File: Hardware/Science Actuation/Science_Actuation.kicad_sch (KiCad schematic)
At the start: 110 parts, among them J2 RJ45_LED_Shielded, Q1 BSS138, Q10 AO3401A, Q9 BSS138, SW1 SW_Push, SW10 SW_SPDT, SW2 SW_Push, SW3 SW_Push, SW4 SW_Push, SW5 SW_Push, SW6 SW_Push, SW7 SW_Push, SW8 SW_Push, SW9 SW_Push, U2 OKI, U2 Teensy4.1_DEV-16771

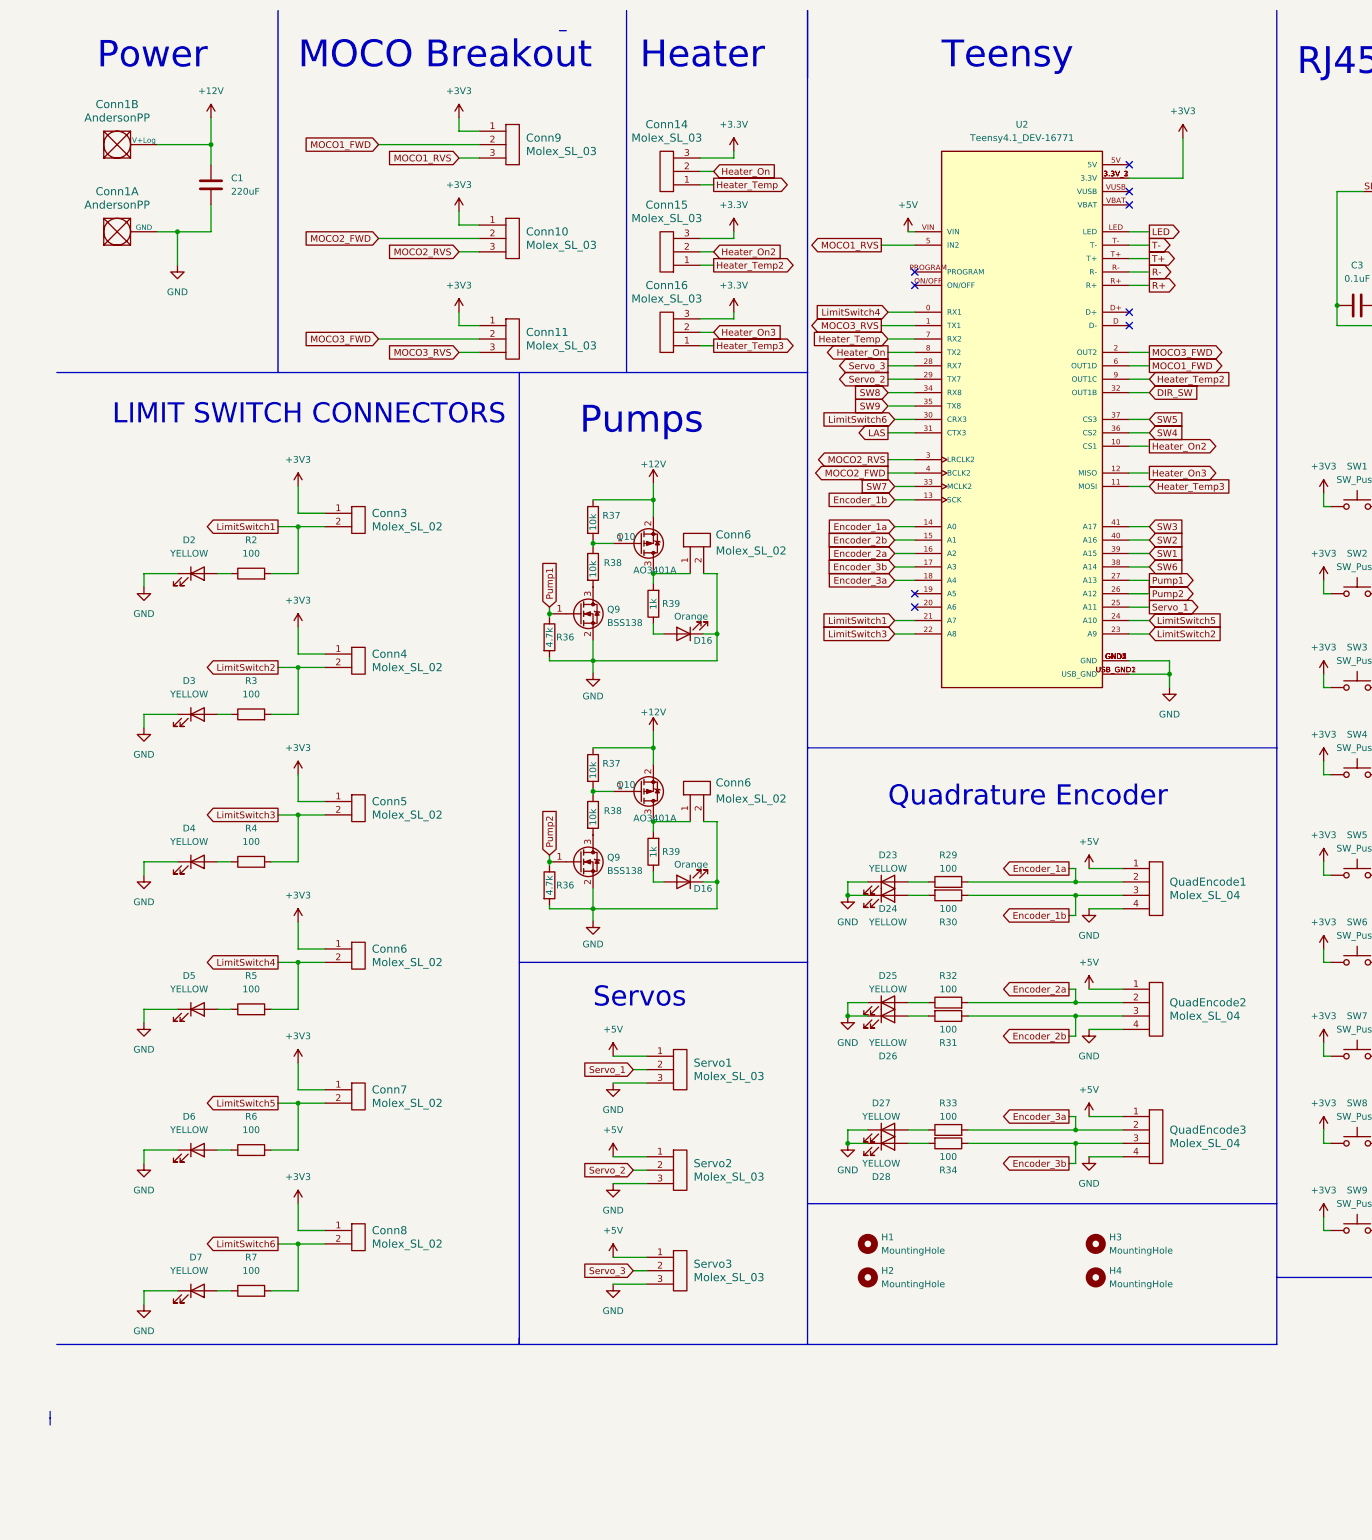
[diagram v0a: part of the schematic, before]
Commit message: Temporary state
Removed things. Added a motor. WIP
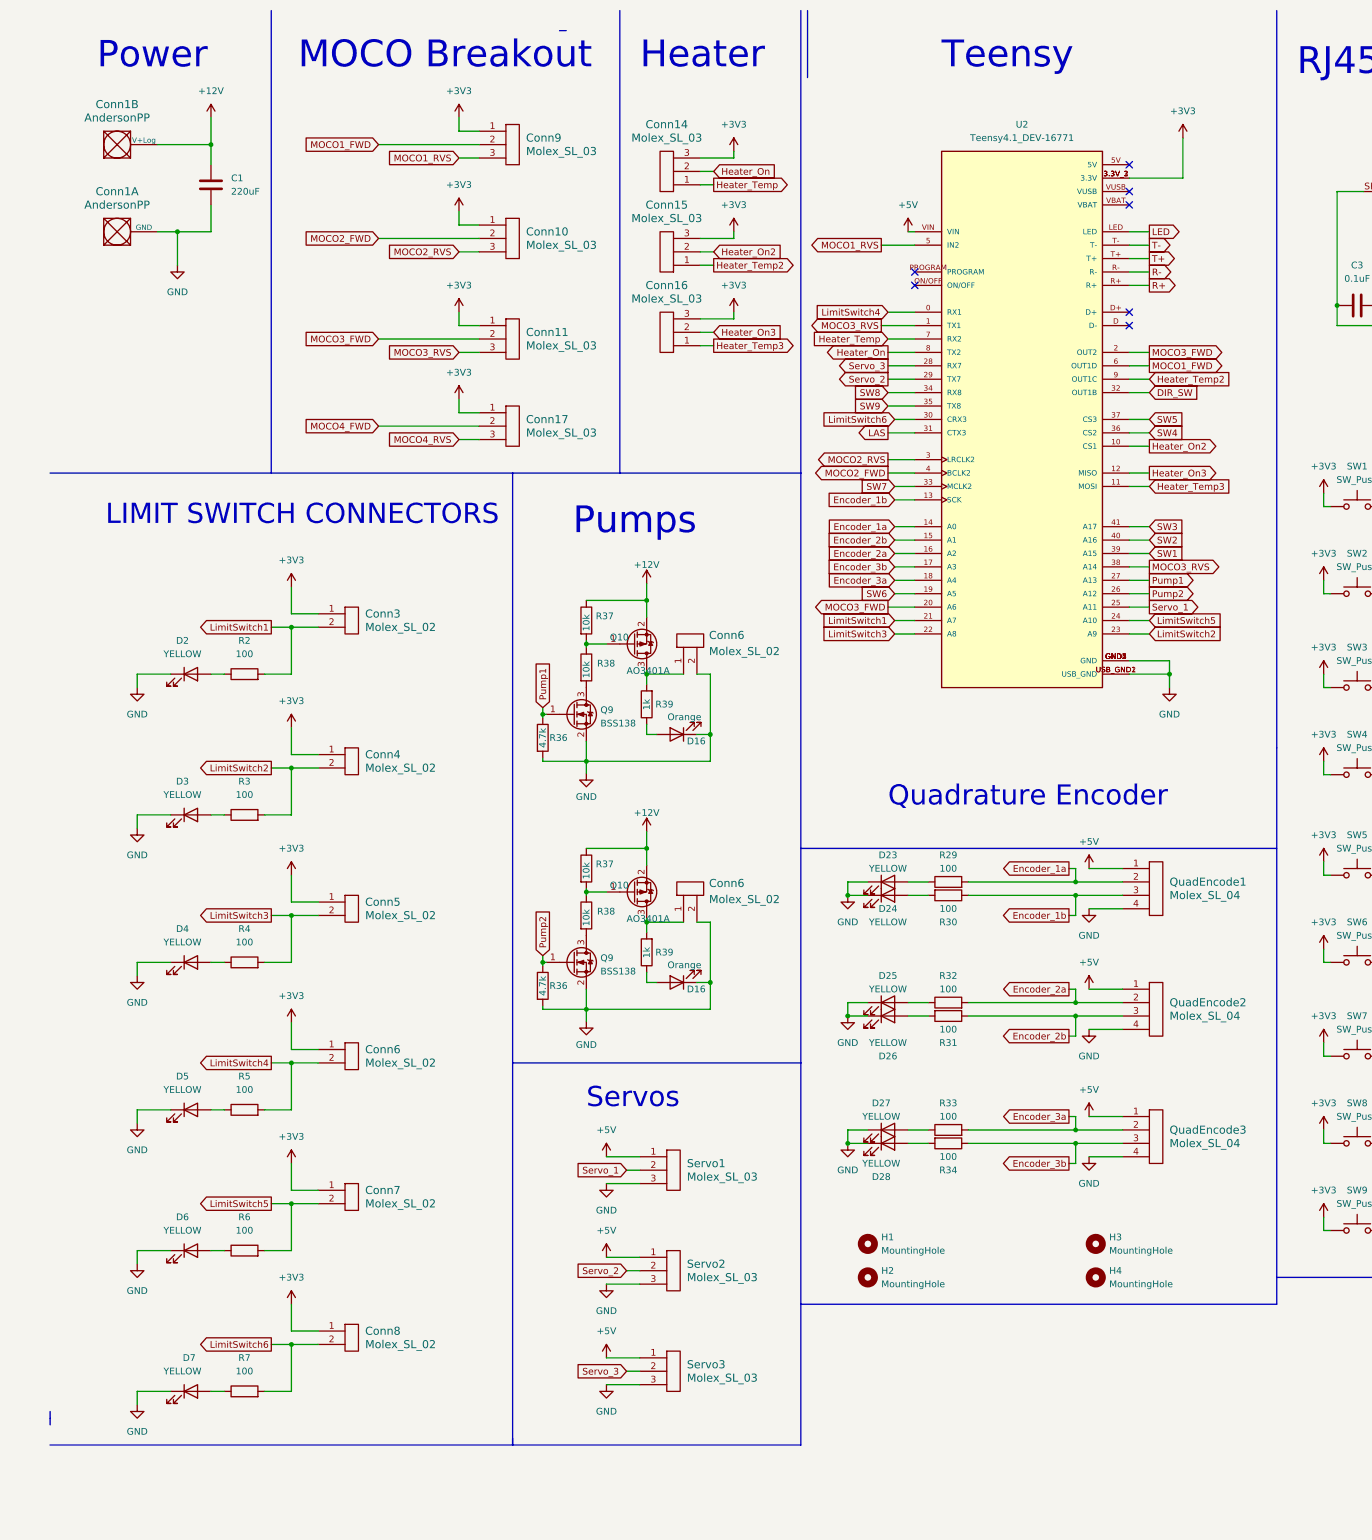
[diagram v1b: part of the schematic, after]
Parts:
- added Conn17: Molex_SL_03, MRDT_Connectors:MOLEX_SL_03_Vertical, symbol MRDT_Connectors:Molex_SL_03
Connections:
- net +3.3V is gone; now on net +3V3: Conn14.3, Conn15.3, Conn16.3
- net +3V3: now also Conn17.1
- net MOCO3_FWD: now also U2.20 (A6)
- net MOCO3_RVS: now also U2.38 (A14)
- net Pump1: no longer Q9.1 (G), R36.1, U2.26 (A12)
- net SW6: now also U2.19 (A5); no longer U2.38 (A14)
- new net MOCO4_FWD: Conn17.2
- new net MOCO4_RVS: Conn17.3
- new net Pump2: Q9.1 (G), R36.1, U2.26 (A12)
- no-connect marks 12 -> 10
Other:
- moved on the sheet: Conn3, Conn4, Conn5, Conn6, Conn7, Conn8, D16, D2, D3, D4, D5, D6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
